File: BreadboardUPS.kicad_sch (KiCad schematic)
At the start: 4 parts, among them J101 Conn_01x04_Pin, J102 Conn_01x02_Pin, J103 Conn_01x02_Pin

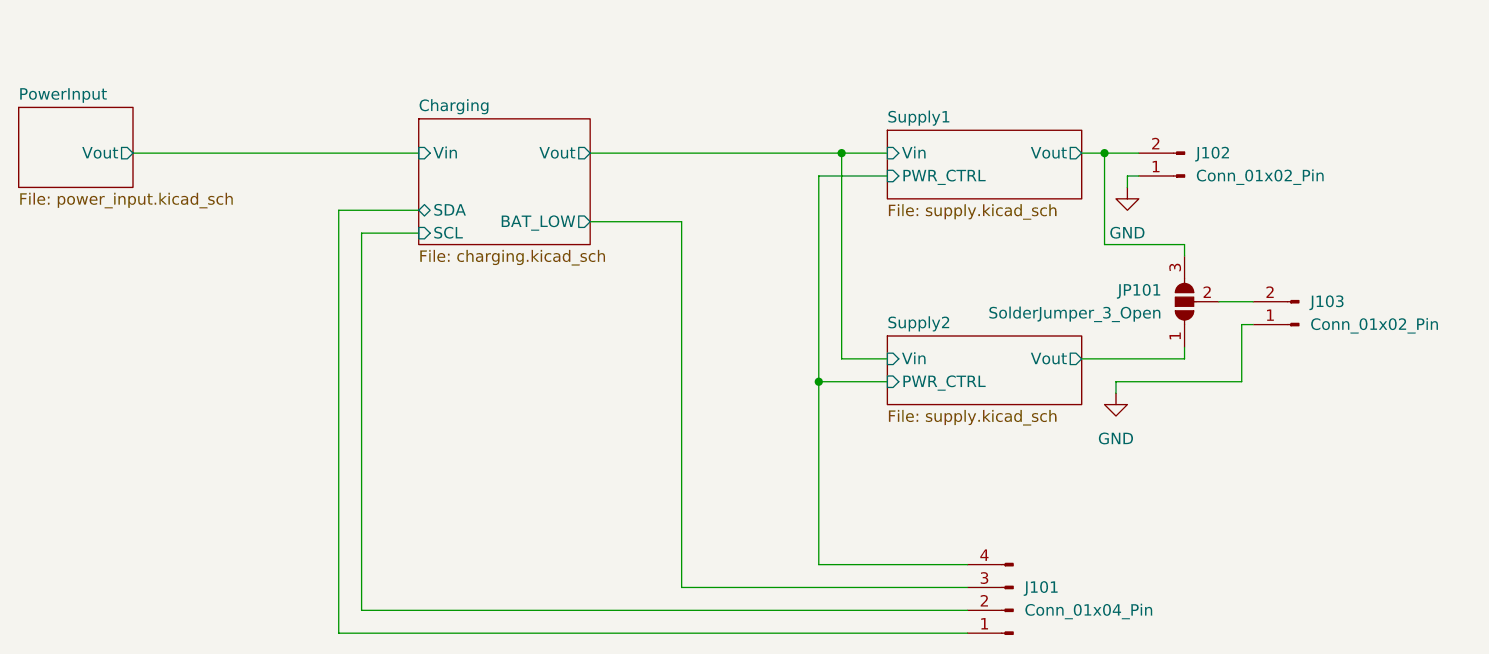
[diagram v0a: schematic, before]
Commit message: Connection naming
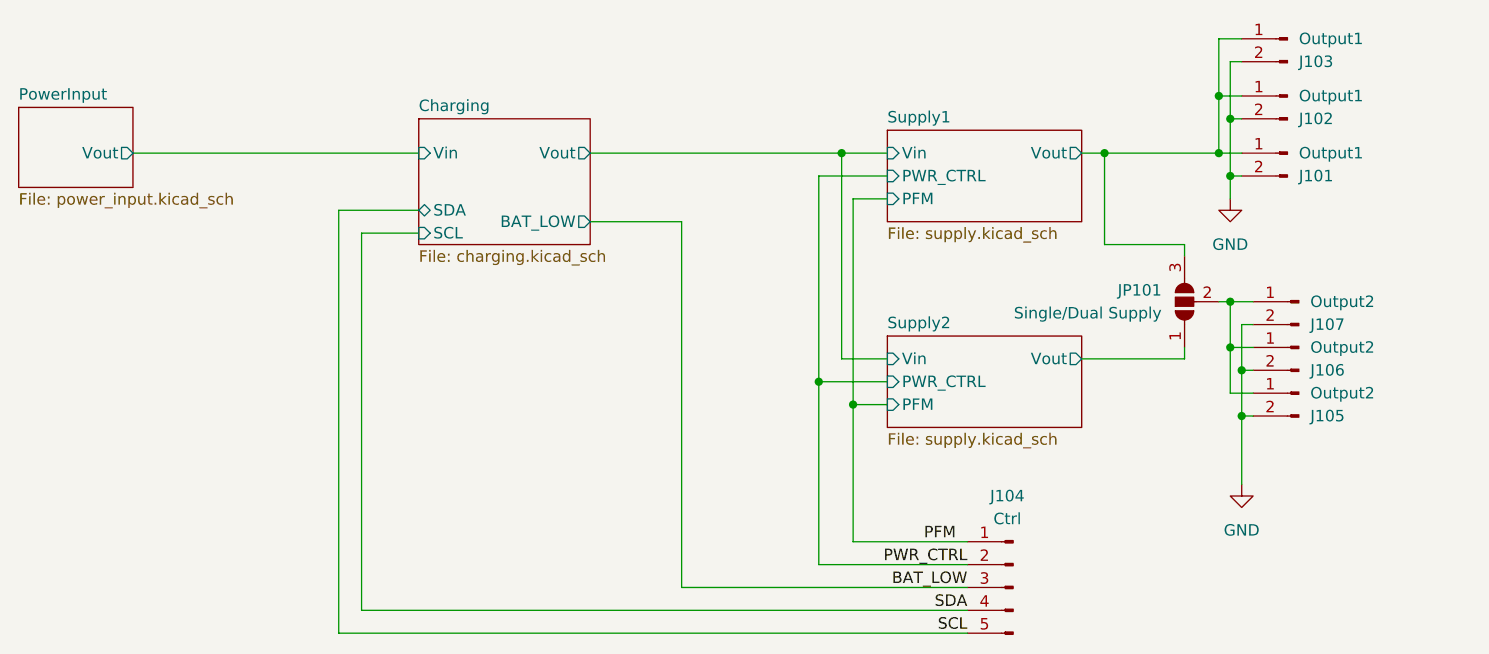
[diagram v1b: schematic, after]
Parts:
- removed J101: Conn_01x04_Pin, Connector_PinHeader_2.54mm:PinHeader_1x04_P2.54mm_Vertical, symbol Connector:Conn_01x04_Pin
- added J101: Output1, Connector_PinHeader_2.54mm:PinHeader_1x02_P2.54mm_Vertical, symbol Connector:Conn_01x02_Pin
- added J104: Ctrl, Connector_PinHeader_2.54mm:PinHeader_1x05_P2.54mm_Vertical, symbol Connector:Conn_01x05_Pin
- added J105, J106, J107: Output2, Connector_PinHeader_2.54mm:PinHeader_1x02_P2.54mm_Vertical, symbol Connector:Conn_01x02_Pin
- J102, J103: value Conn_01x02_Pin -> Output1
- JP101: value SolderJumper_3_Open -> Single/Dual Supply
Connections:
- net GND: now also J102.2 (Pin_2), J103.2 (Pin_2), J101.2 (Pin_2), J105.2 (Pin_2), J106.2 (Pin_2), J107.2 (Pin_2); no longer J102.1 (Pin_1), J103.1 (Pin_1)
- net Supply1/Vout: now also J102.1 (Pin_1), J103.1 (Pin_1), J101.1 (Pin_1); no longer J102.2 (Pin_2)
- net at JP101.2 (C): now also J105.1 (Pin_1), J106.1 (Pin_1), J107.1 (Pin_1); no longer J103.2 (Pin_2)
- new net BAT_LOW: J104.3 (Pin_3)
- new net PFM: J104.1 (Pin_1)
- new net PWR_CTRL: J104.2 (Pin_2)
- new net SCL: J104.5 (Pin_5)
- new net SDA: J104.4 (Pin_4)
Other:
- sheet Supply1 ports: added PFM; removed none
- sheet Supply2 ports: added PFM; removed none
